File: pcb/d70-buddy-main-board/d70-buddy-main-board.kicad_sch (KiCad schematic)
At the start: 12 parts, among them J1 PJ-327C-4A, J2 PJ-327C-4A, J3 Conn_02x12_Top_Bottom, U1 H11L1, U2 Pico

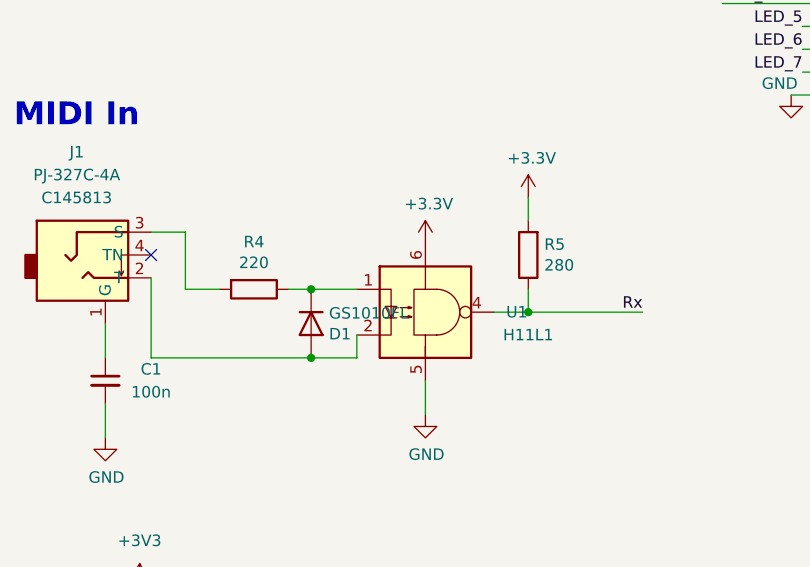
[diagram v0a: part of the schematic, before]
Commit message: Wip
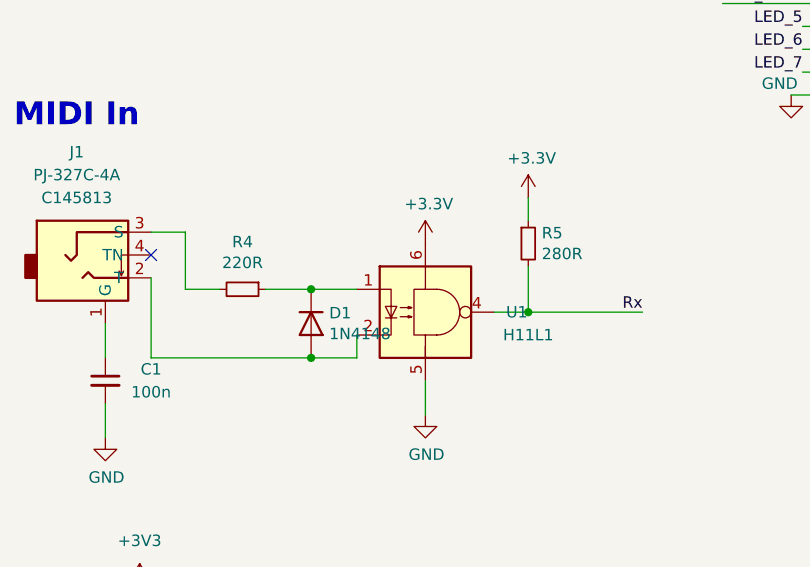
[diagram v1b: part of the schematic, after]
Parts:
- removed D1: GS1010FL, Diodes_SMD:D_SOD-123F, symbol Device:D
- removed R4: 220, Resistors_SMD:R_0603_HandSoldering, symbol Device:R
- removed R5: 280, Resistors_SMD:R_0603_HandSoldering, symbol Device:R
- added D1: 1N4148, Diode_SMD:D_0805_2012Metric, symbol Diode:1N4148
- added R4: 220R, Resistor_SMD:R_0402_1005Metric, symbol Device:R_Small
- added R5: 280R, Resistor_SMD:R_0402_1005Metric, symbol Device:R_Small
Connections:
- net +3V3: now also R5.1
- net Rx: now also R5.2
- net at U1.1: now also D1.1 (K), R4.1
- net at J1.2 (T), U1.2: now also D1.2 (A)
- net at J1.3 (S): now also R4.2
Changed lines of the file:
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@@
   (junction (at 153.67 73.66) (diameter 0) (color 0 0 0 0)
   )
+  (junction (at 62.23 77.47) (diameter 0) (color 0 0 0 0)
+  )
+  (junction (at 212.09 78.74) (diameter 0) (color 0 0 0 0)
+  )
   (junction (at 62.23 85.09) (diameter 0) (color 0 0 0 0)
-  )
-  (junction (at 212.09 78.74) (diameter 0) (color 0 0 0 0)
-  )
-  (junction (at 62.23 77.47) (diameter 0) (color 0 0 0 0)
   )
   (junction (at 43.18 110.49) (diameter 0) (color 0 0 0 0)
@@
     (stroke (width 0) (type default) (color 0 0 0 0))
   )
+  (wire (pts (xy 154.94 88.9) (xy 162.56 88.9))
+    (stroke (width 0) (type default) (color 0 0 0 0))
+  )
+  (wire (pts (xy 52.07 77.47) (xy 48.26 77.47))
+    (stroke (width 0) (type default) (color 0 0 0 0))
+  )
+  (wire (pts (xy 107.95 35.56) (xy 119.38 35.56))
+    (stroke (width 0) (type default) (color 0 0 0 0))
+  )
+  (wire (pts (xy 198.12 104.14) (xy 207.01 104.14))
+    (stroke (width 0) (type default) (color 0 0 0 0))
+  )
+  (wire (pts (xy 44.45 85.09) (xy 62.23 85.09))
+    (stroke (width 0) (type default) (color 0 0 0 0))
+  )
+  (wire (pts (xy 86.36 74.93) (xy 86.36 80.01))
+    (stroke (width 0) (type default) (color 0 0 0 0))
+  )
+  (wire (pts (xy 207.01 111.76) (xy 198.12 111.76))
+    (stroke (width 0) (type default) (color 0 0 0 0))
+  )
+  (wire (pts (xy 39.37 90.17) (xy 39.37 93.98))
+    (stroke (width 0) (type default) (color 0 0 0 0))
+  )
+  (wire (pts (xy 132.08 27.94) (xy 148.59 27.94))
+    (stroke (width 0) (type default) (color 0 0 0 0))
+  )
+  (wire (pts (xy 43.18 121.92) (xy 50.8 121.92))
+    (stroke (width 0) (type default) (color 0 0 0 0))
+  )
+  (wire (pts (xy 113.03 38.1) (xy 119.38 38.1))
+    (stroke (width 0) (type default) (color 0 0 0 0))
+  )
+  (wire (pts (xy 205.74 116.84) (xy 198.12 116.84))
+    (stroke (width 0) (type default) (color 0 0 0 0))
+  )
   (wire (pts (xy 62.23 85.09) (xy 67.31 85.09))
     (stroke (width 0) (type default) (color 0 0 0 0))
   )
-  (wire (pts (xy 154.94 88.9) (xy 162.56 88.9))
-    (stroke (width 0) (type default) (color 0 0 0 0))
-  )
-  (wire (pts (xy 52.07 77.47) (xy 48.26 77.47))
-    (stroke (width 0) (type default) (color 0 0 0 0))
-  )
-  (wire (pts (xy 107.95 35.56) (xy 119.38 35.56))
-    (stroke (width 0) (type default) (color 0 0 0 0))
-  )
-  (wire (pts (xy 198.12 104.14) (xy 207.01 104.14))
-    (stroke (width 0) (type default) (color 0 0 0 0))
-  )
-  (wire (pts (xy 44.45 85.09) (xy 62.23 85.09))
-    (stroke (width 0) (type default) (color 0 0 0 0))
-  )
-  (wire (pts (xy 207.01 111.76) (xy 198.12 111.76))
-    (stroke (width 0) (type default) (color 0 0 0 0))
-  )
-  (wire (pts (xy 39.37 90.17) (xy 39.37 93.98))
-    (stroke (width 0) (type default) (color 0 0 0 0))
-  )
-  (wire (pts (xy 86.36 77.47) (xy 86.36 80.01))
-    (stroke (width 0) (type default) (color 0 0 0 0))
-  )
-  (wire (pts (xy 132.08 27.94) (xy 148.59 27.94))
-    (stroke (width 0) (type default) (color 0 0 0 0))
-  )
-  (wire (pts (xy 43.18 121.92) (xy 50.8 121.92))
-    (stroke (width 0) (type default) (color 0 0 0 0))
-  )
-  (wire (pts (xy 113.03 38.1) (xy 119.38 38.1))
-    (stroke (width 0) (type default) (color 0 0 0 0))
-  )
-  (wire (pts (xy 205.74 116.84) (xy 198.12 116.84))
-    (stroke (width 0) (type default) (color 0 0 0 0))
-  )
   (wire (pts (xy 203.2 93.98) (xy 198.12 93.98))
     (stroke (width 0) (type default) (color 0 0 0 0))
@@
     (stroke (width 0) (type default) (color 0 0 0 0))
   )
+  (wire (pts (xy 57.15 77.47) (xy 62.23 77.47))
+    (stroke (width 0) (type default) (color 0 0 0 0))
+  )
   (wire (pts (xy 203.2 68.58) (xy 198.12 68.58))
     (stroke (width 0) (type default) (color 0 0 0 0))
   )
   (wire (pts (xy 86.36 80.01) (xy 82.55 80.01))
-    (stroke (width 0) (type default) (color 0 0 0 0))
-  )
-  (wire (pts (xy 59.69 77.47) (xy 62.23 77.47))
     (stroke (width 0) (type default) (color 0 0 0 0))
   )
@@
     (pin "9")
   )
-  (symbol (lib_id "Device:R") (at 86.36 73.66 180) (unit 1)
-    (in_bom yes) (on_board yes)
-    (property "Reference" "R5" (id 0) (at 88.138 72.4916 0)
-      (effects (font (size 1.27 1.27)) (justify right))
-    )
-    (property "Value" "280" (id 1) (at 88.138 74.803 0)
-      (effects (font (size 1.27 1.27)) (justify right))
-    )
-    (property "Footprint" "Resistors_SMD:R_0603_HandSoldering" (id 2) (at 88.138 73.66 90)
-      (effects (font (size 1.27 1.27)) hide)
-    )
-    (property "Datasheet" "~" (id 3) (at 86.36 73.66 0)
-      (effects (font (size 1.27 1.27)) hide)
-    )
-    (pin "1")
-    (pin "2")
-  )
   (symbol (lib_id "power:GND") (at 207.01 111.76 0) (unit 1)
     (in_bom yes) (on_board yes)
@@
     (pin "2")
   )
-  (symbol (lib_id "Device:D") (at 62.23 81.28 270) (unit 1)
-    (in_bom yes) (on_board yes)
-    (property "Reference" "D1" (id 0) (at 64.2112 82.4484 90)
-      (effects (font (size 1.27 1.27)) (justify left))
-    )
-    (property "Value" "GS1010FL" (id 1) (at 64.2112 80.137 90)
-      (effects (font (size 1.27 1.27)) (justify left))
-    )
-    (property "Footprint" "Diodes_SMD:D_SOD-123F" (id 2) (at 62.23 81.28 0)
-      (effects (font (size 1.27 1.27)) hide)
-    )
-    (property "Datasheet" "~" (id 3) (at 62.23 81.28 0)
-      (effects (font (size 1.27 1.27)) hide)
-    )
-    (pin "1")
-    (pin "2")
-  )
   (symbol (lib_id "power:GND") (at 148.59 27.94 0) (mirror y) (unit 1)
     (in_bom yes) (on_board yes)
@@
     (pin "1")
   )
+  (symbol (lib_id "Device:R_Small") (at 54.61 77.47 270) (unit 1)
+    (in_bom yes) (on_board yes)
+    (property "Reference" "R4" (id 0) (at 54.61 72.2122 90))
+    (property "Value" "220R" (id 1) (at 54.61 74.5236 90))
+    (property "Footprint" "Resistor_SMD:R_0402_1005Metric" (id 2) (at 54.61 75.692 90)
+      (effects (font (size 1.27 1.27)) hide)
+    )
+    (property "Datasheet" "~" (id 3) (at 54.61 77.47 0)
+      (effects (font (size 1.27 1.27)) hide)
+    )
+    (property "Mouser" " 667-ERJ-6ENF2200V " (id 4) (at 54.61 77.47 0)
+      (effects (font (size 1.27 1.27)) hide)
+    )
+    (pin "1")
+    (pin "2")
+  )
   (symbol (lib_id "power:GND") (at 115.57 55.88 0) (mirror y) (unit 1)
     (in_bom yes) (on_board yes)
@@
     (pin "1")
   )
+  (symbol (lib_id "Diode:1N4148") (at 62.23 81.28 270) (unit 1)
+    (in_bom yes) (on_board yes)
+    (property "Reference" "D1" (id 0) (at 64.2366 80.1116 90)
+      (effects (font (size 1.27 1.27)) (justify left))
+    )
+    (property "Value" "1N4148" (id 1) (at 64.2366 82.423 90)
+      (effects (font (size 1.27 1.27)) (justify left))
+    )
+    (property "Footprint" "Diode_SMD:D_0805_2012Metric" (id 2) (at 57.785 81.28 0)
+      (effects (font (size 1.27 1.27)) hide)
+    )
+    (property "Datasheet" "https://assets.nexperia.com/documents/data-sheet/1N4148_1N4448.pdf" (id 3) (at 62.23 81.28 0)
+      (effects (font (size 1.27 1.27)) hide)
+    )
+    (pin "1")
+    (pin "2")
+  )
   (symbol (lib_id "power:GND") (at 74.93 91.44 0) (unit 1)
     (in_bom yes) (on_board yes)
@@
     )
     (pin "1")
+  )
+  (symbol (lib_id "Device:R_Small") (at 86.36 72.39 0) (unit 1)
+    (in_bom yes) (on_board yes)
+    (property "Reference" "R5" (id 0) (at 87.8586 71.2216 0)
+      (effects (font (size 1.27 1.27)) (justify left))
+    )
+    (property "Value" "280R" (id 1) (at 87.8586 73.533 0)
+      (effects (font (size 1.27 1.27)) (justify left))
+    )
+    (property "Footprint" "Resistor_SMD:R_0402_1005Metric" (id 2) (at 86.36 72.39 0)
+      (effects (font (size 1.27 1.27)) hide)
+    )
+    (property "Datasheet" "~" (id 3) (at 86.36 72.39 0)
+      (effects (font (size 1.27 1.27)) hide)
+    )
+    (property "Mouser" " 667-ERJ-6ENF1002V " (id 4) (at 86.36 72.39 0)
+      (effects (font (size 1.27 1.27)) hide)
+    )
+    (pin "1")
+    (pin "2")
   )
   (symbol (lib_id "power:GND") (at 210.82 86.36 0) (unit 1)
@@
     (pin "4")
   )
-  (symbol (lib_id "Device:R") (at 55.88 77.47 270) (unit 1)
-    (in_bom yes) (on_board yes)
-    (property "Reference" "R4" (id 0) (at 55.88 72.2122 90))
-    (property "Value" "220" (id 1) (at 55.88 74.5236 90))
-    (property "Footprint" "Resistors_SMD:R_0603_HandSoldering" (id 2) (at 55.88 75.692 90)
-      (effects (font (size 1.27 1.27)) hide)
-    )
-    (property "Datasheet" "~" (id 3) (at 55.88 77.47 0)
-      (effects (font (size 1.27 1.27)) hide)
-    )
-    (pin "1")
-    (pin "2")
-  )
   (sheet_instances
     (path "/" (page "1"))
@@
       (reference "C1") (unit 1) (value "100n") (footprint "Capacitor_SMD:C_0402_1005Metric")
     )
-    (path "/5125c4d9-cf5c-4fe5-9dc8-c939e40fcd6f"
-      (reference "D1") (unit 1) (value "GS1010FL") (footprint "Diodes_SMD:D_SOD-123F")
+    (path "/cb435343-5406-4ba5-9c93-0ff71089b3d2"
+      (reference "D1") (unit 1) (value "1N4148") (footprint "Diode_SMD:D_0805_2012Metric")
     )
     (path "/f8941761-7033-4bbc-b902-69429032853d"
@@
       (reference "R3") (unit 1) (value "68R") (footprint "Resistor_SMD:R_0402_1005Metric")
     )
-    (path "/f9570ec9-4338-4208-aee7-369a45a284f8"
-      (reference "R4") (unit 1) (value "220") (footprint "Resistors_SMD:R_0603_HandSoldering")
-    )
-    (path "/12c9f3e1-9431-42f8-b6f8-fb6fd35fc1cb"
-      (reference "R5") (unit 1) (value "280") (footprint "Resistors_SMD:R_0603_HandSoldering")
+    (path "/c208ca27-6451-4b64-a11c-ed1d60333bed"
+      (reference "R4") (unit 1) (value "220R") (footprint "Resistor_SMD:R_0402_1005Metric")
+    )
+    (path "/dbaff88d-b9b2-4076-872a-6f6dec25038b"
+      (reference "R5") (unit 1) (value "280R") (footprint "Resistor_SMD:R_0402_1005Metric")
     )
     (path "/9678c00c-6ef4-4c2b-a3b2-09bd5a765528"
